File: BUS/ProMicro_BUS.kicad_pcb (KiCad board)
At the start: 2 copper layers, 17.8 x 30.5 mm, 17 parts, among them J1 Conn_01x03, U1 MAX3483, U2 MCP2515-xSO, U3 MAX3051, Y1 Crystal

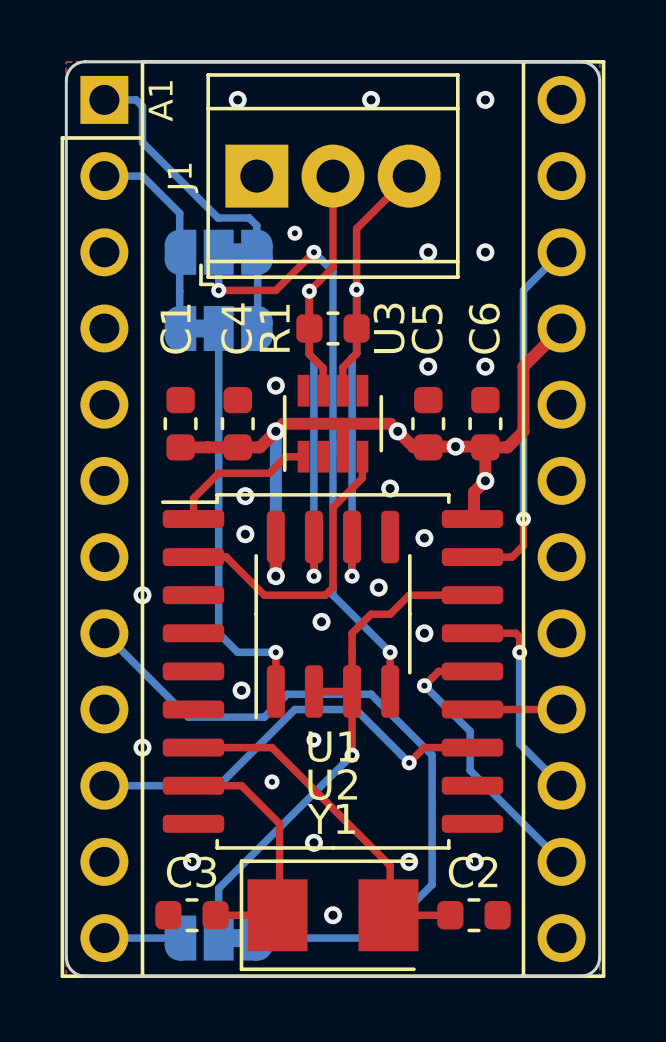
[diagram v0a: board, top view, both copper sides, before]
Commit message: dump
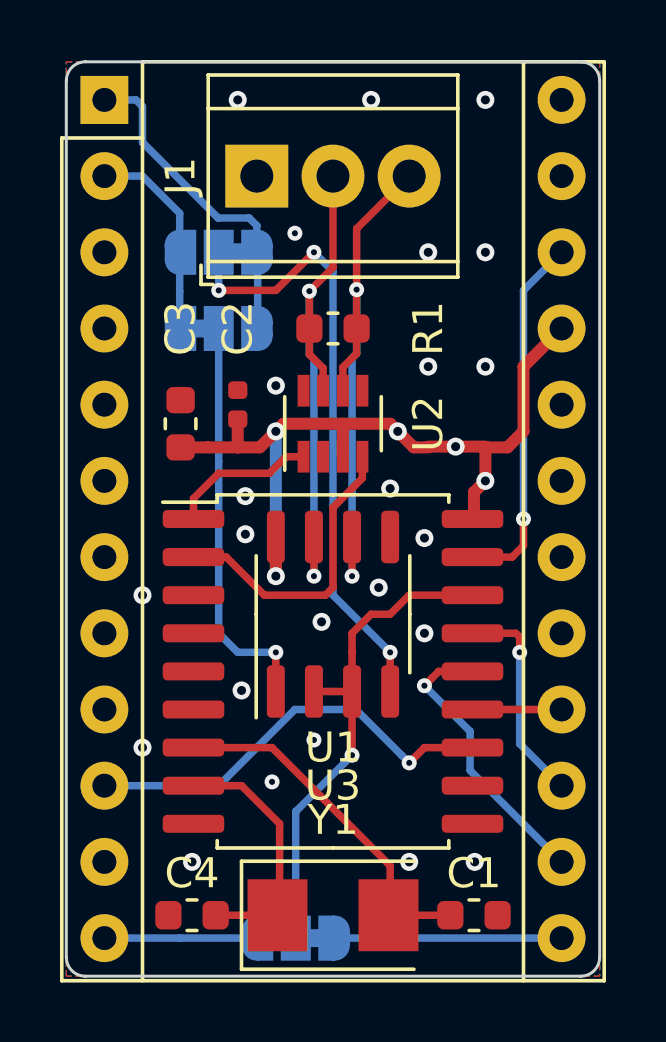
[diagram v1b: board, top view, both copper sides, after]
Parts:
- removed the C1 at (53.3, 87.0)
- removed the C4 at (55.2, 87.0)
- removed C5, C6: 100n, Capacitor_SMD:C_0603_1608Metric
- added C2: 100n, Capacitor_SMD:C_0402_1005Metric, F.Cu at (55.2, 86.4)
- added C3: 10µ, Capacitor_SMD:C_0603_1608Metric, F.Cu at (53.3, 87.0)
- A1: value Sparkfun_Pro_Micro_3V3 -> Sparkfun_Pro_Micro
- moved LOGO1 10.4 mm to (59.1, 100.3), turned to 90 degrees
- moved JP3 2.57 mm to (57.2, 104.1)
- renumbered C2 to C1, C3 to C4, JP2 to JP1, JP1 to JP2, U3 to U2, U2 to U3
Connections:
- net D0 renamed TXD
- net D1 renamed RXD
- net D14 renamed CIPO
- net D15 renamed SCK
- net D16 renamed COPI
- net D7 renamed INT
- net D9 renamed CS1
- net Reset renamed ~RST
- A1 pad 13: (no net) -> CS0
- A1 pad 8: D5 -> (no net)
- JP3 pad 1: D5 -> CS0
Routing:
- net D5: track 24.1 -> 0.00 mm
- net CS0: track 0.00 -> 7.56 mm
- net CS1: track 2.51 -> 5.08 mm
- net CS: track 17.6 -> 16.6 mm
- net +3V3: track 26.1 -> 27.0 mm
- net GND: vias 26 -> 24
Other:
- board text added: "A"
- board text added: "B"
- board text added: "CIPO"
- board text added: "COPI"
- board text added: "CS0"
- board text added: "CS1"
- board text added: "G"
- board text added: "nerdyscout.github.io/ ProMicro/BUS v1.3"
- board text added: "~RST"
- board text removed: "CS"
- board text removed: "MISO"
- board text removed: "MOSI"
- board text removed: "RESET"
- board text removed: "TXDEN"
- board text removed: "nerdyscout.github.io/ProMicro/BUS"
- board text removed: "v1.2"
